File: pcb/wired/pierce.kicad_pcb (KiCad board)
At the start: 2 copper layers, 115 x 91.4 mm, 37 parts, among them SW11 SW_PUSH, SW12 SW_PUSH, SW13 SW_PUSH, SW14 SW_PUSH, SW19 SW_PUSH, SW20 SW_PUSH, SW21 SW_PUSH, SW22 SW_PUSH, SW27 SW_PUSH, SW28 SW_PUSH, SW29 SW_PUSH, SW34 SW_PUSH, SW35 SW_PUSH, SW36 SW_PUSH, SW4 SW_PUSH, SW5 SW_PUSH, SW6 SW_PUSH, SW7 SW_PUSH

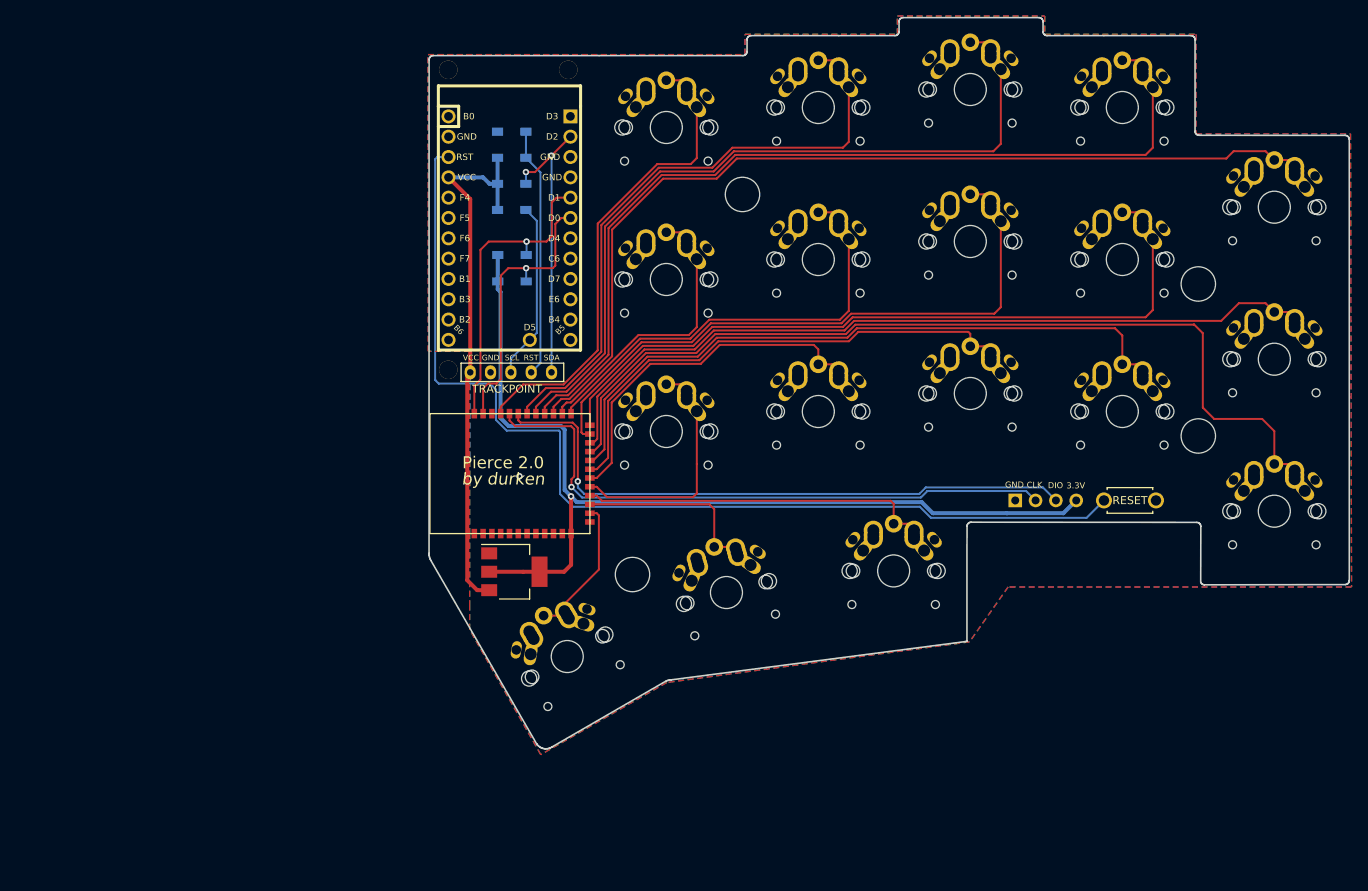
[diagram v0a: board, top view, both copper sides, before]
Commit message: prototype - ordered
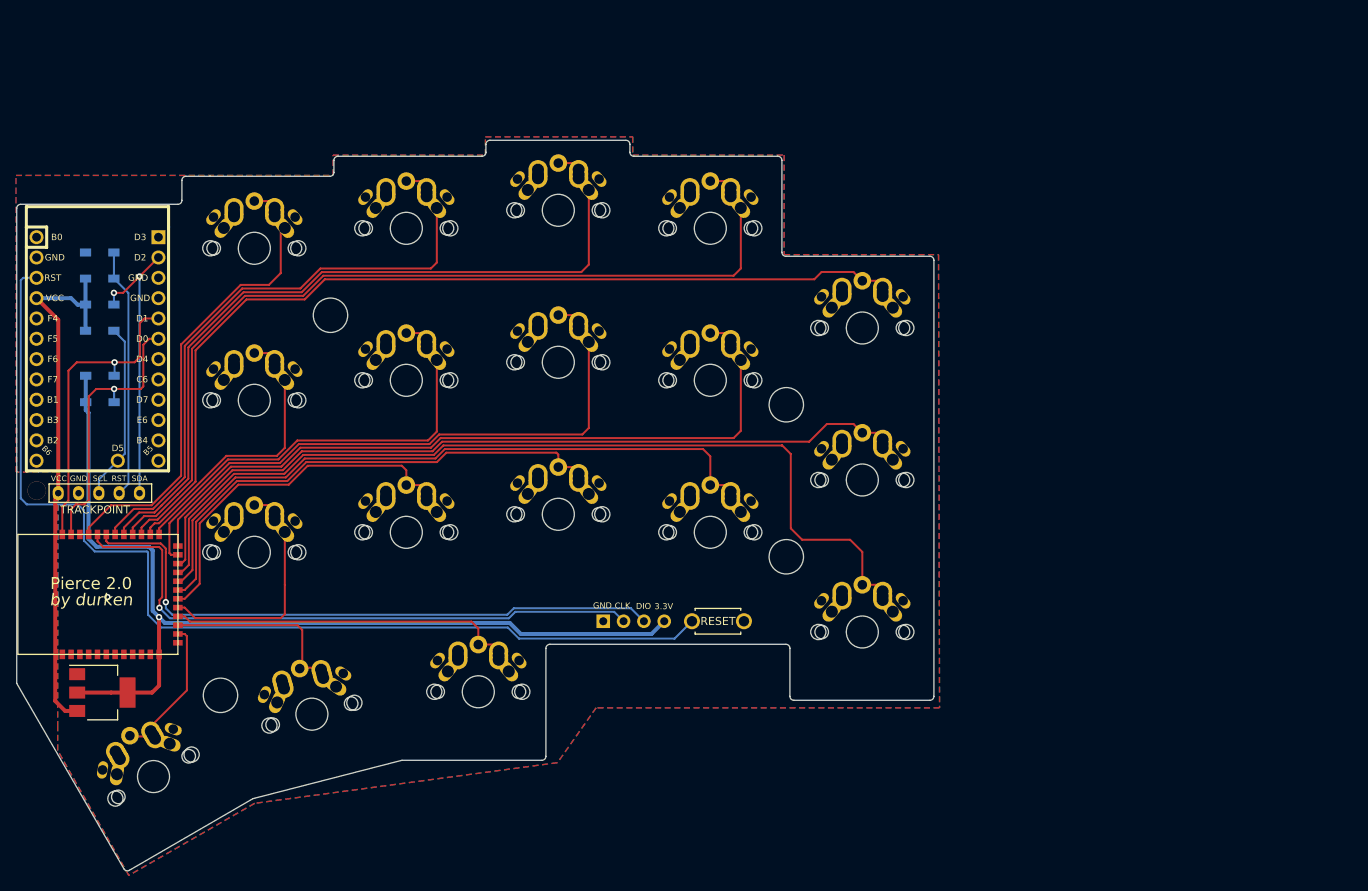
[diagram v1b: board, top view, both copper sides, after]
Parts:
- removed the Ref** at (164.5, 30.5)
- removed the Ref** at (149.5, 30.5)
- moved SW22 54.1 mm to (153.3, 108.2)
- moved SW14 54.0 mm to (132.5, 111.0)
- moved SW7 53.8 mm to (112.7, 118.8)
- moved AVR1 53.7 mm to (105.4, 65.4)
- moved REG1 53.7 mm to (106.3, 108.3)
- moved Ref** 53.7 mm to (121.0, 108.7)
- moved SW13 53.7 mm to (144.3, 88.3)
- moved SW20 53.7 mm to (163.3, 67.1)
- moved SW21 53.7 mm to (163.3, 86.1)
- moved SW35 53.7 mm to (201.3, 81.8)
- moved SW36 53.7 mm to (201.3, 100.8)
- moved SW4 53.7 mm to (125.3, 52.8)
- moved SW5 53.7 mm to (125.3, 71.8)
- moved SW6 53.7 mm to (125.3, 90.8)
- moved TP1 53.7 mm to (100.7, 83.4)
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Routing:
- net SW32R: track 45.8 -> 45.1 mm
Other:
- board size 115 x 91.4 mm -> 114.6 x 91.3 mm
- net class Default removed
